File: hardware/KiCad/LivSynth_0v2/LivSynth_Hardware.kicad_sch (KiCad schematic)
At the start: 0 parts

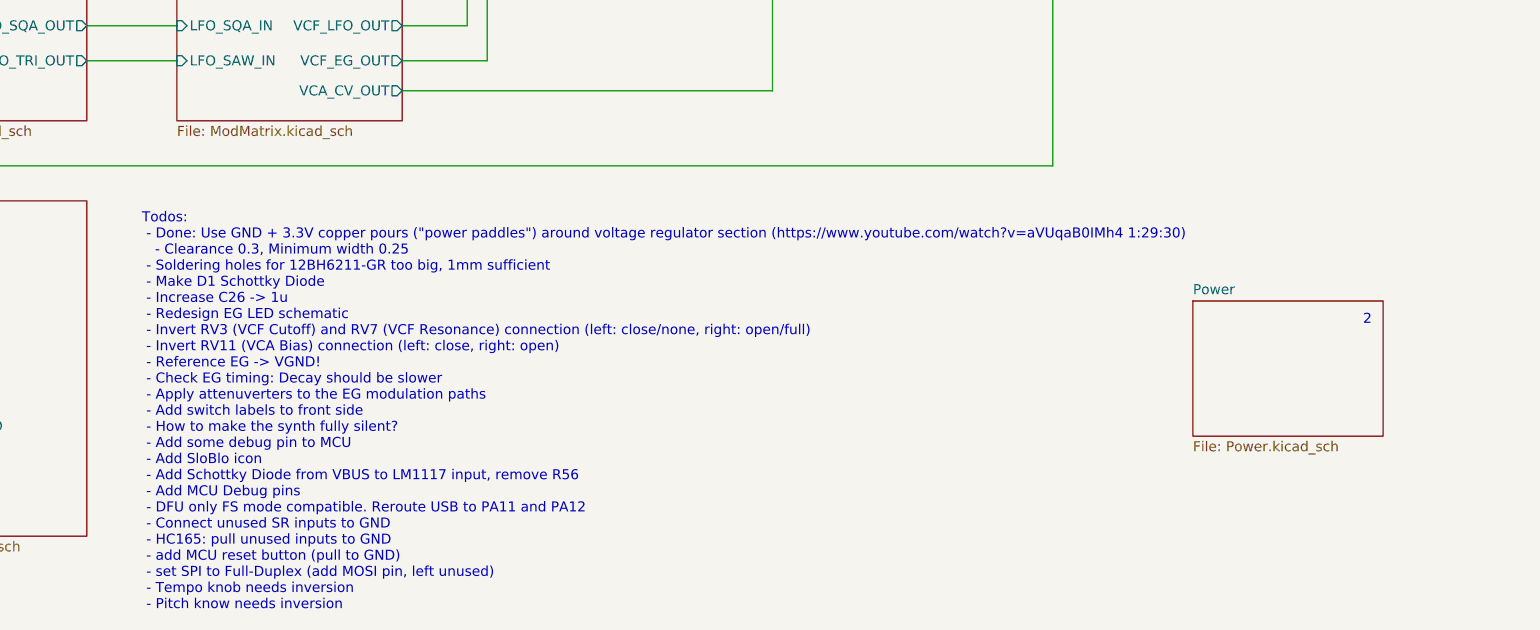
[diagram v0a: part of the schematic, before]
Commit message: Before fixing HW issues
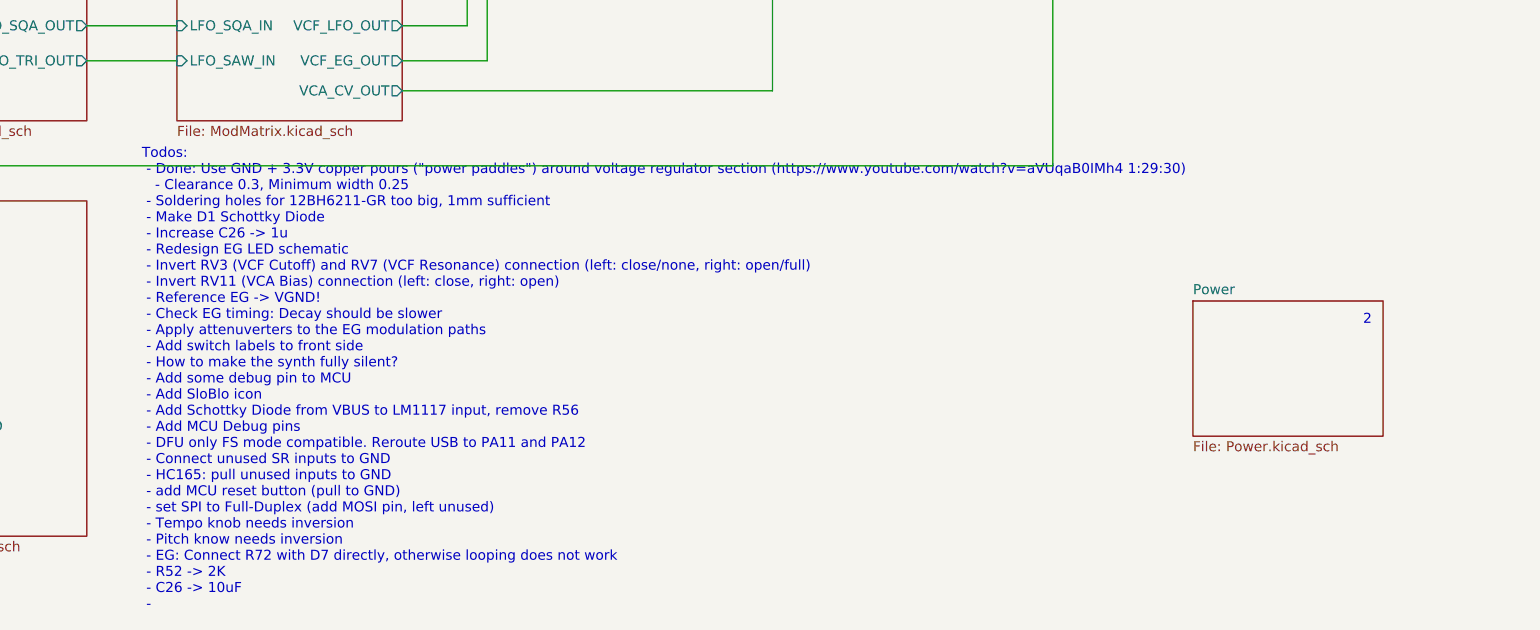
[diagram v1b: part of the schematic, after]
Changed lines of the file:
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@@
     (effects (font (size 1.27 1.27)) (justify left bottom))
   )
-  (text "Todos:\n - Done: Use GND + 3.3V copper pours (\"power paddles\") around voltage regulator section (https://www.youtube.com/watch?v=aVUqaB0IMh4 1:29:30)\n   - Clearance 0.3, Minimum width 0.25\n - Soldering holes for 12BH6211-GR too big, 1mm sufficient\n - Make D1 Schottky Diode\n - Increase C26 -> 1u\n - Redesign EG LED schematic\n - Invert RV3 (VCF Cutoff) and RV7 (VCF Resonance) connection (left: close/none, right: open/full)\n - Invert RV11 (VCA Bias) connection (left: close, right: open)\n - Reference EG -> VGND!\n - Check EG timing: Decay should be slower\n - Apply attenuverters to the EG modulation paths\n - Add switch labels to front side\n - How to make the synth fully silent?\n - Add some debug pin to MCU\n - Add SloBlo icon\n - Add Schottky Diode from VBUS to LM1117 input, remove R56\n - Add MCU Debug pins\n - DFU only FS mode compatible. Reroute USB to PA11 and PA12\n - Connect unused SR inputs to GND\n - HC165: pull unused inputs to GND\n - add MCU reset button (pull to GND)\n - set SPI to Full-Duplex (add MOSI pin, left unused)\n - Tempo knob needs inversion\n - Pitch know needs inversion\n"
+  (text "Todos:\n - Done: Use GND + 3.3V copper pours (\"power paddles\") around voltage regulator section (https://www.youtube.com/watch?v=aVUqaB0IMh4 1:29:30)\n   - Clearance 0.3, Minimum width 0.25\n - Soldering holes for 12BH6211-GR too big, 1mm sufficient\n - Make D1 Schottky Diode\n - Increase C26 -> 1u\n - Redesign EG LED schematic\n - Invert RV3 (VCF Cutoff) and RV7 (VCF Resonance) connection (left: close/none, right: open/full)\n - Invert RV11 (VCA Bias) connection (left: close, right: open)\n - Reference EG -> VGND!\n - Check EG timing: Decay should be slower\n - Apply attenuverters to the EG modulation paths\n - Add switch labels to front side\n - How to make the synth fully silent?\n - Add some debug pin to MCU\n - Add SloBlo icon\n - Add Schottky Diode from VBUS to LM1117 input, remove R56\n - Add MCU Debug pins\n - DFU only FS mode compatible. Reroute USB to PA11 and PA12\n - Connect unused SR inputs to GND\n - HC165: pull unused inputs to GND\n - add MCU reset button (pull to GND)\n - set SPI to Full-Duplex (add MOSI pin, left unused)\n - Tempo knob needs inversion\n - Pitch know needs inversion\n - EG: Connect R72 with D7 directly, otherwise looping does not work\n - R52 -> 2K\n - C26 -> 10uF\n - "
     (at 120.65 182.88 0)
     (effects (font (size 1.27 1.27)) (justify left bottom))
@@
     )
     (path "/5bba0015-9baa-48b8-b961-e7169713a149/5bcd4196-1721-40ea-bafe-95ac02171038"
-      (reference "R34") (unit 1) (value "20K") (footprint "Resistor_THT:R_Axial_DIN0207_L6.3mm_D2.5mm_P7.62mm_Horizontal")
+      (reference "R34") (unit 1) (value "4K7") (footprint "Resistor_THT:R_Axial_DIN0207_L6.3mm_D2.5mm_P7.62mm_Horizontal")
     )
     (path "/a0830201-d177-4d04-9261-1bfa7e92760e/f8eadc45-80ee-4534-a705-4c60e25b1d15"
